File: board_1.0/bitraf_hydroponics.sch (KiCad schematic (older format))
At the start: 40 parts, among them P1 12V, P10 I2C_4, P11 BUZZER, P12 LDR, P13 TEMP_HUM, P14 PROGRAMMER, P15 SPI, P16 RADIO_433, P2 SWITCH_1, P3 SWITCH_2, P4 SWITCH_3, P5 LCD, P6 ROT_ENC, P7 I2C_1, P8 I2C_2, P9 I2C_3, Q1 DMN2041L-7, Q2 DMN2041L-7, Q3 DMN2041L-7, U1 TPS54202, U2 AP2114H-3.3TRG1, U3 ESP-12F

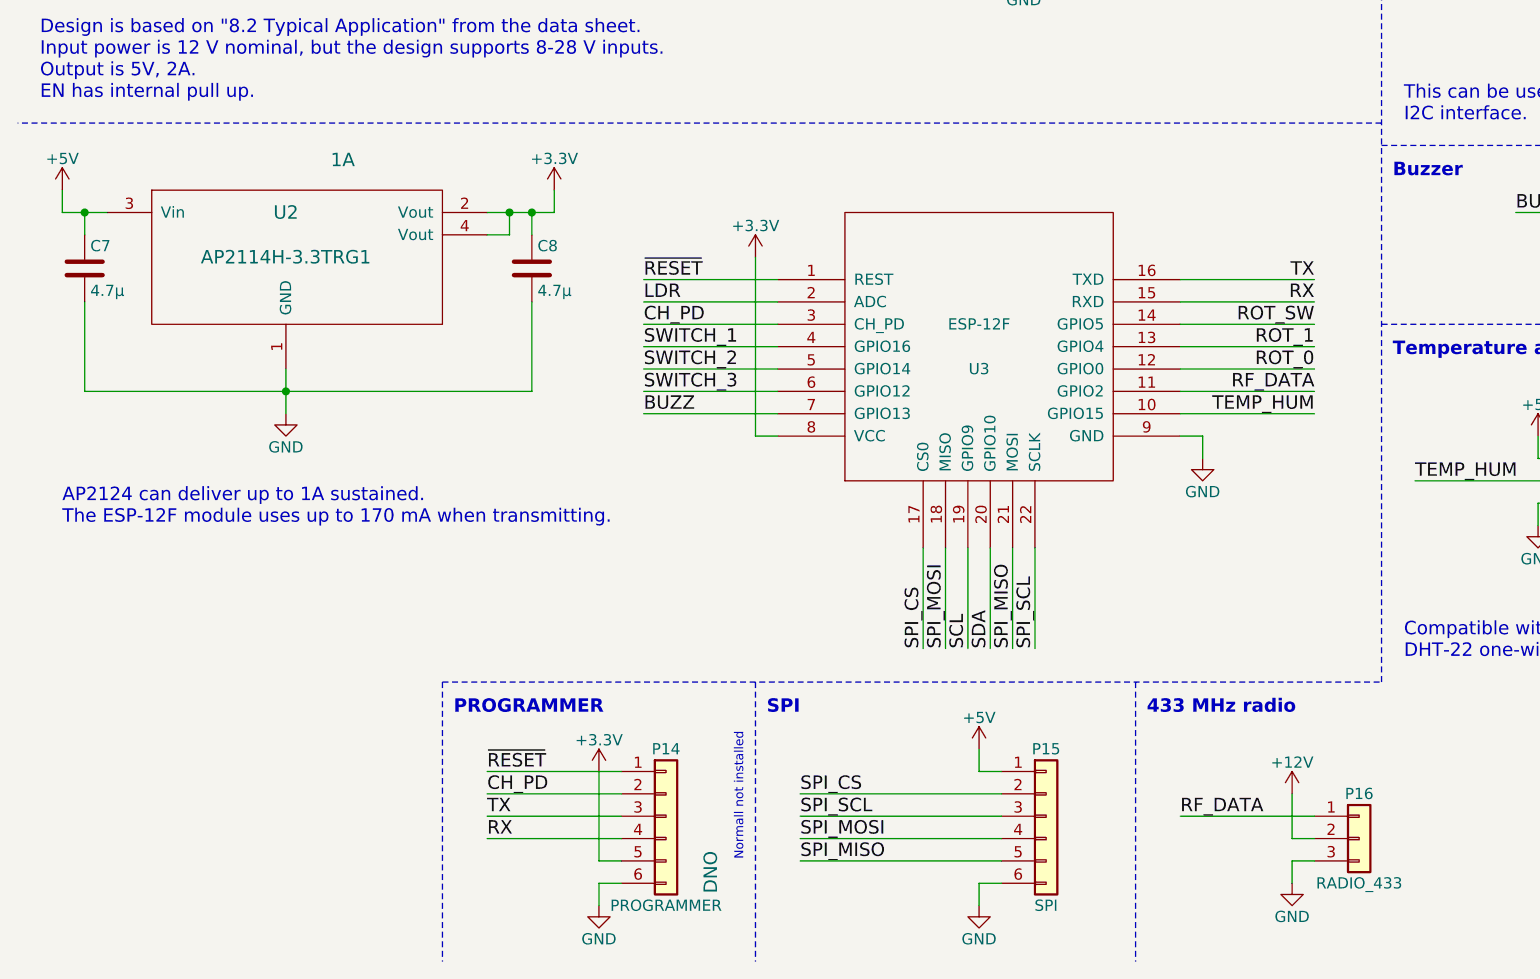
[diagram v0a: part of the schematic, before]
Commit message: Added pullups and jumper header fro programming. Still need to tweak the mosfets, but need expert help
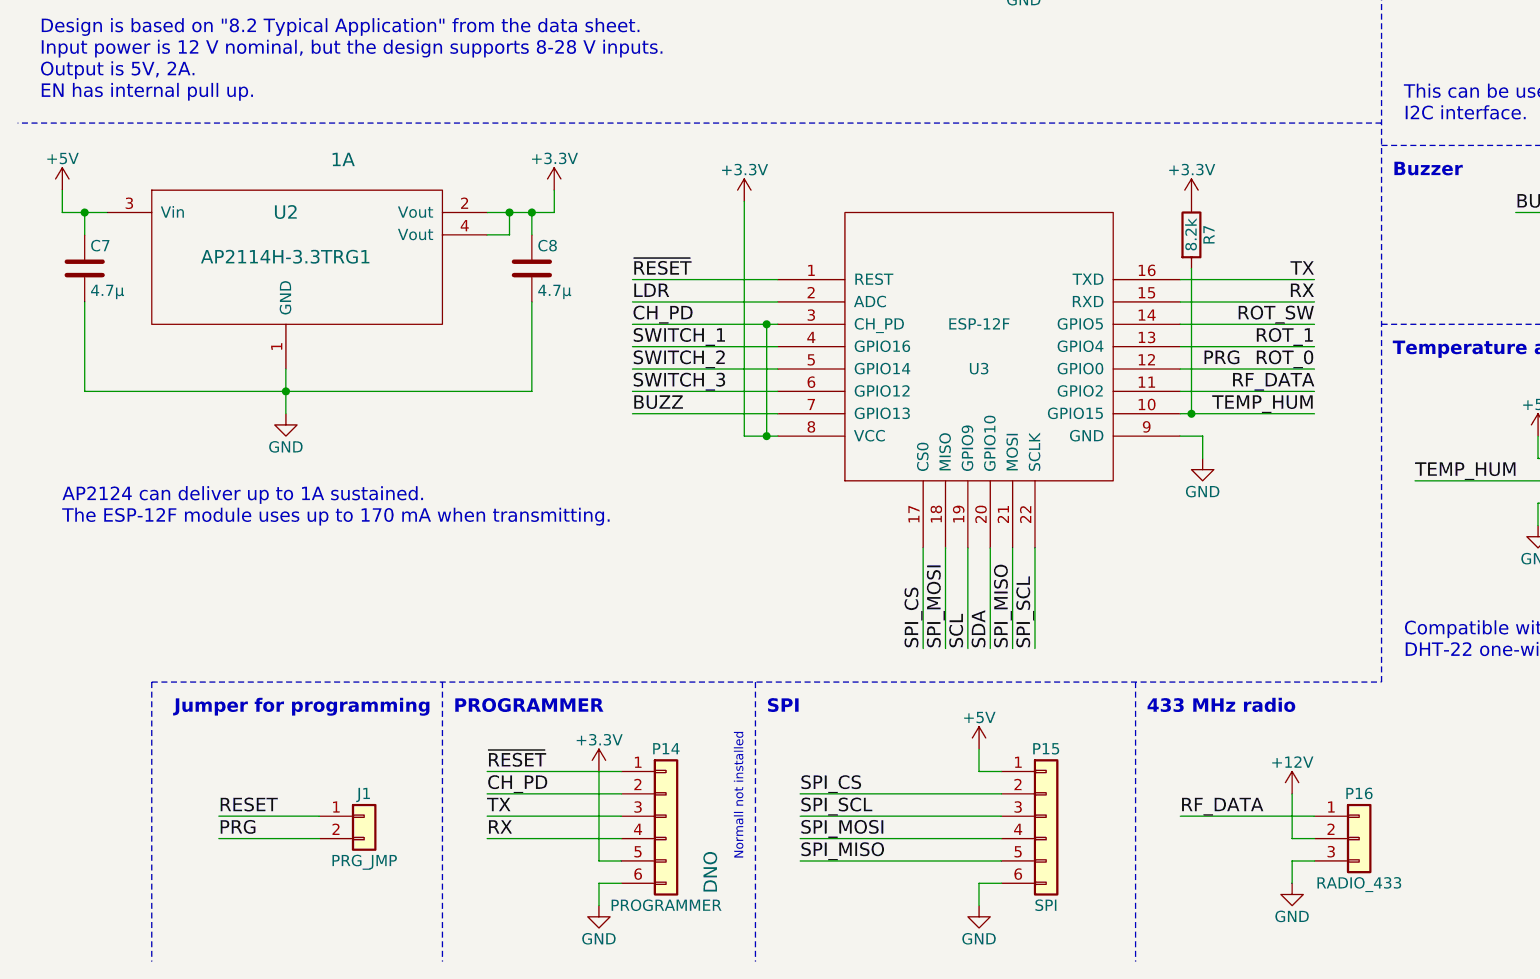
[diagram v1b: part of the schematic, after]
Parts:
- added J1: PRG_JMP, Pin_Headers:Pin_Header_Straight_1x02_Pitch2.54mm, symbol Conn_01x02
- added R7: 8.2k, Resistors_SMD:R_0805, symbol R
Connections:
- net CH_PD is gone; now on net +3V3: P14.2 (Pin_2), U3.3 (CH_PD)
- net +3V3: now also R7.1
- net TEMP_HUM: now also R7.2
- net ROT_0 renamed PRG
- net PRG: now also J1.2 (Pin_2)
- new net RESET: J1.1 (Pin_1)
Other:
- note added: "Jumper for programming"

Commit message: This should go in it's own branch/folder. Revert "Added pullups and jumper header fro programming. Still need to tweak the mosfets, but need expert help"
This reverts commit b0ba335143d29f2dde67b78845eb19ede0b5a3d2.
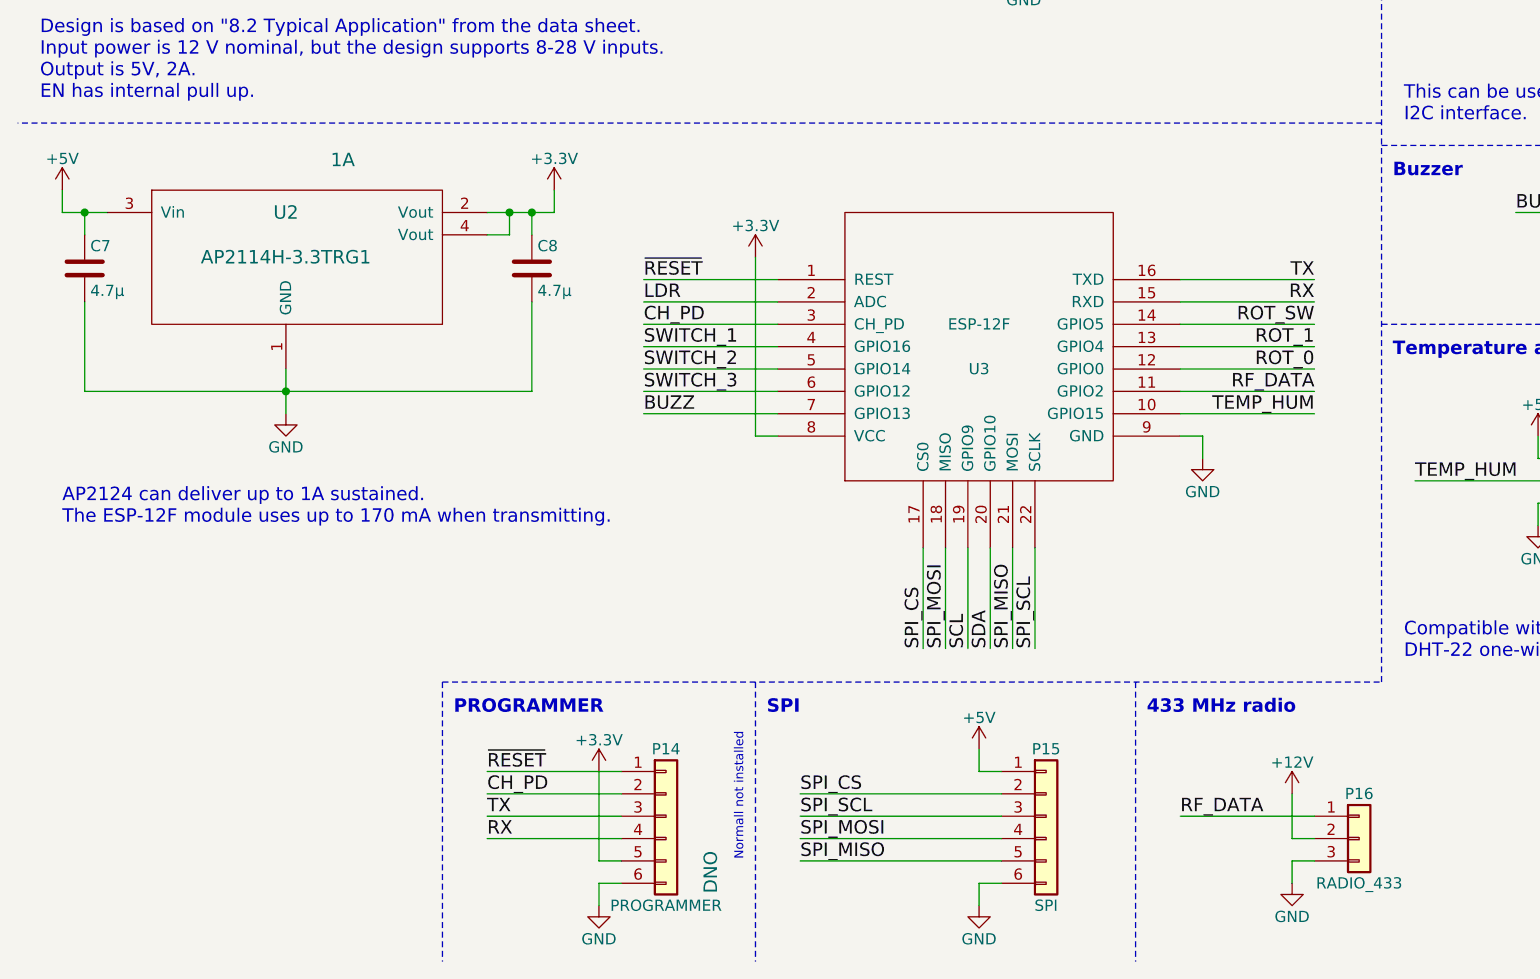
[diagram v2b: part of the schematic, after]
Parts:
- removed J1: PRG_JMP, Pin_Headers:Pin_Header_Straight_1x02_Pitch2.54mm, symbol Conn_01x02
- removed R7: 8.2k, Resistors_SMD:R_0805, symbol R
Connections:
- net +3V3: no longer P14.2 (Pin_2), U3.3 (CH_PD)
- net PRG renamed ROT_0
- new net CH_PD: P14.2 (Pin_2), U3.3 (CH_PD)
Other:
- note removed: "Jumper for programming"
